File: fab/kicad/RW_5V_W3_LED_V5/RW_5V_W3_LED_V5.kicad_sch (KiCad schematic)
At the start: 31 parts, among them J1 Conn_01x08_Pin, J2 Conn_01x08_Pin, Q1 BC337, Q2 BC337, Q3 BC337, Q4 BC337

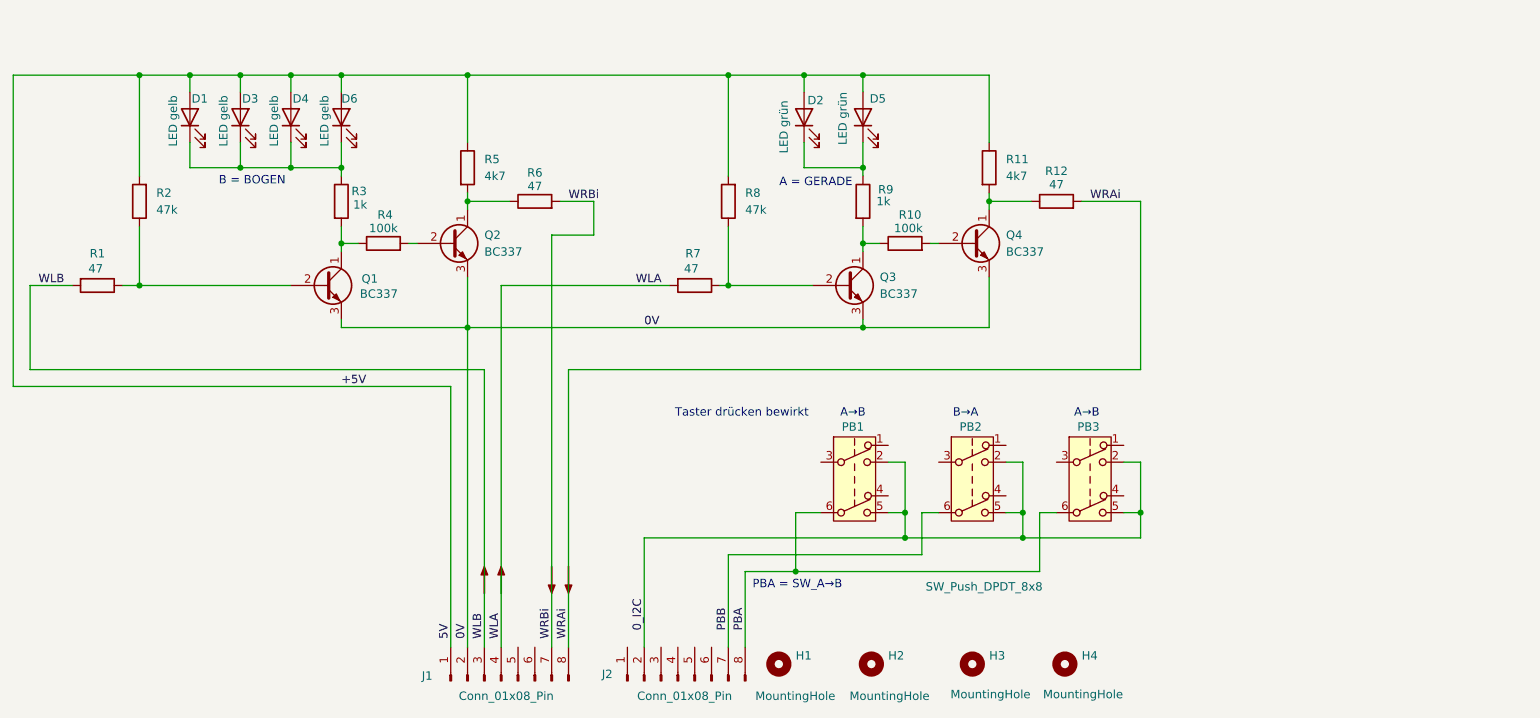
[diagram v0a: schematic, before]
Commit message: Update kicad files
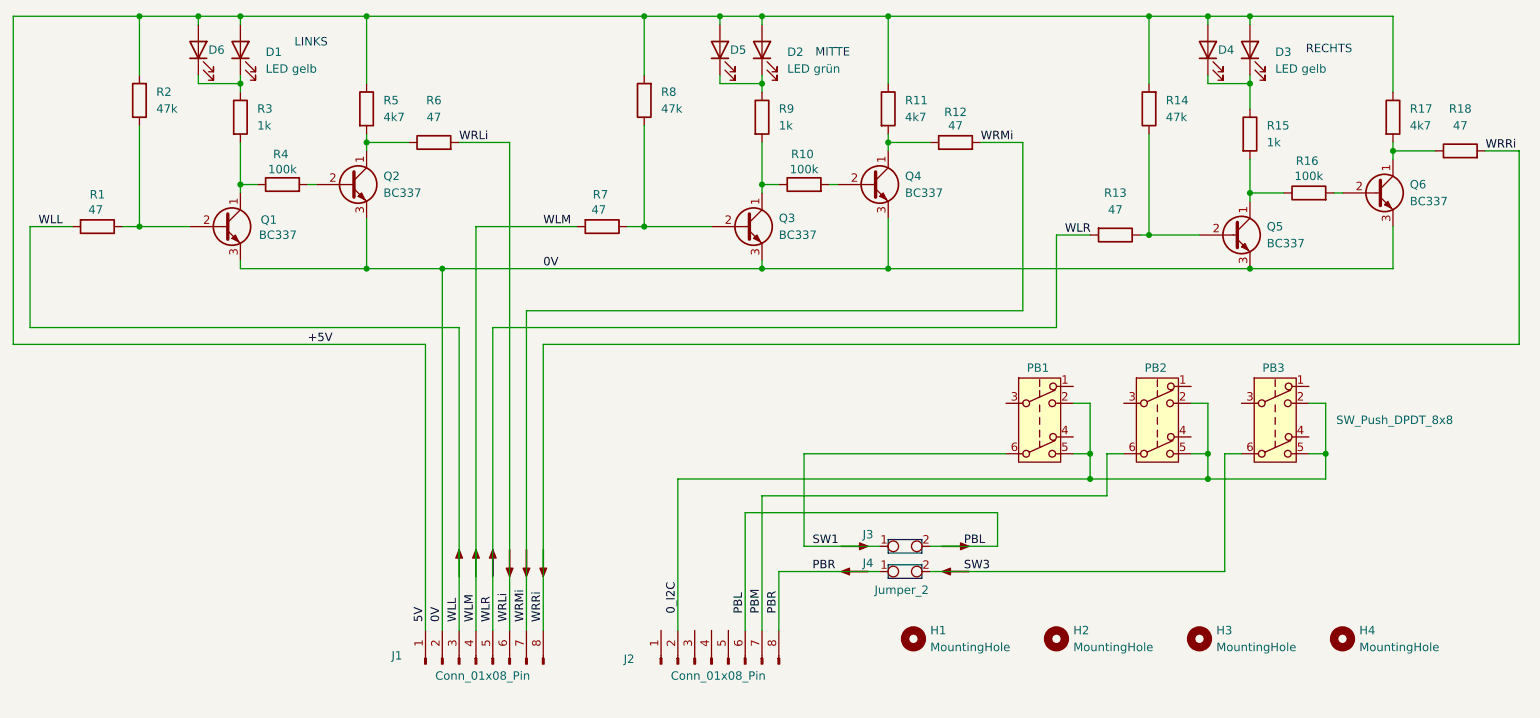
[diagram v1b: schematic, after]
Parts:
- removed D1: LED gelb, LED_THT:LED_D3.0mm, symbol Device:LED
- added D4: LED gelb, _kh_library:LED_D3.0mm_kh, symbol Device:LED
- added J3, J4: Jumper_2, _kh_library:PinSocket_1x02_P2.54mm_Vertical_kh, symbol _kh_library:Jumper_2
- added Q5, Q6: BC337, _kh_library:TO-92_Inline_Wide_custom, symbol Transistor_BJT:BC337
- added R13, R18: 47, Resistor_THT:R_Axial_DIN0204_L3.6mm_D1.6mm_P2.54mm_Vertical, symbol Device:R
- added R14: 47k, Resistor_THT:R_Axial_DIN0204_L3.6mm_D1.6mm_P2.54mm_Vertical, symbol Device:R
- added R15: 1k, Resistor_THT:R_Axial_DIN0204_L3.6mm_D1.6mm_P2.54mm_Vertical, symbol Device:R
- added R16: 100k, _kh_library:R_Axial_DIN0204_L3.6mm_D1.6mm_P3.81mm_Vertical_kh, symbol Device:R
- added R17: 4k7, Resistor_THT:R_Axial_DIN0204_L3.6mm_D1.6mm_P2.54mm_Vertical, symbol Device:R
- D1: renamed from D6; footprint LED_THT:LED_D3.0mm -> _kh_library:LED_D3.0mm_kh
- D2: renamed from D5; footprint LED_THT:LED_D3.0mm -> _kh_library:LED_D3.0mm_kh
- D3: footprint LED_THT:LED_D3.0mm -> _kh_library:LED_D3.0mm_kh
- D5: renamed from D2; footprint LED_THT:LED_D3.0mm -> _kh_library:LED_D3.0mm_kh
- D6: renamed from D4; footprint LED_THT:LED_D3.0mm -> _kh_library:LED_D3.0mm_kh
- J1, J2: footprint _kh_library:PinSocket_1x08_P2.54mm_Vertical_kh -> _kh_library:PinSocket_1x08_P2.54mm_Vertical_11mm_kh
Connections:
- net +5V: now also D4.2 (A), R14.2, R17.1
- net 0V: now also Q5.3 (E), Q6.3 (E)
- net at D1.1 (K), D6.1 (K), R3.1: no longer D3.1 (K)
- net PBL: now reaches J2.6 (Pin_6)
- net PBL: now also J3.2 (Pin_2)
- net WLR: now reaches J1.5 (Pin_5)
- net WLR: now also R13.2
- net WRLi: now reaches J1.6 (Pin_6)
- net WRLi: now also R6.2
- removed net PBA: J2.8 (Pin_8), PB1.6 (C), PB3.6 (C)
- net PBB renamed PBM
- net WLA renamed WLM
- net WLB renamed WLL
- net WRAi renamed WRMi
- net WRMi: now also J1.7 (Pin_7); no longer J1.8 (Pin_8)
- removed net WRBi: J1.7 (Pin_7), R6.2
- new net: Q6.1 (C), R17.2, R18.1
- new net: Q5.2 (B), R13.1, R14.1
- new net: D3.1 (K), D4.1 (K), R15.1
- new net: Q5.1 (C), R15.2, R16.1
- new net: Q6.2 (B), R16.2
- new net PBR: J2.8 (Pin_8), J4.1 (Pin_1)
- new net SW1: J3.1 (Pin_1), PB1.6 (C)
- new net SW3: J4.2 (Pin_2), PB3.6 (C)
- new net WRRi: J1.8 (Pin_8), R18.2
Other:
- note added: "LINKS"
- note added: "MITTE"
- note added: "RECHTS"
- note removed: "A = GERADE"
- note removed: "A→B"
- note removed: "B = BOGEN"
- note removed: "B→A"
- note removed: "PBA = SW_A→B"
- note removed: "Taster drücken bewirkt"
- moved on the sheet: D1, D2, D5, D6, H1, H2, H3, H4, J1, J2, PB1, PB2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
